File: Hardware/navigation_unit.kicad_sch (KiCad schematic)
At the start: 34 parts, among them SW1 SW_SPDT, SW2 SW_Push_Dual, U4 STM32F405RGTx, Y1 25MHz

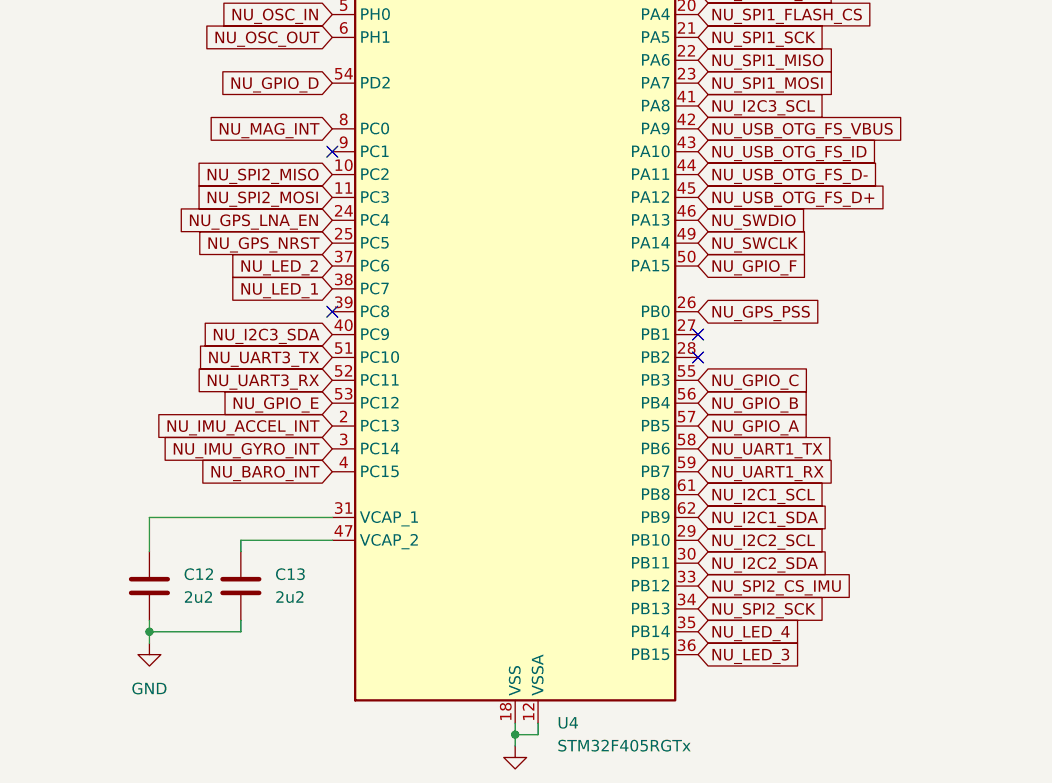
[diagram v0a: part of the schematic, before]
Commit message: i2c sensors traces
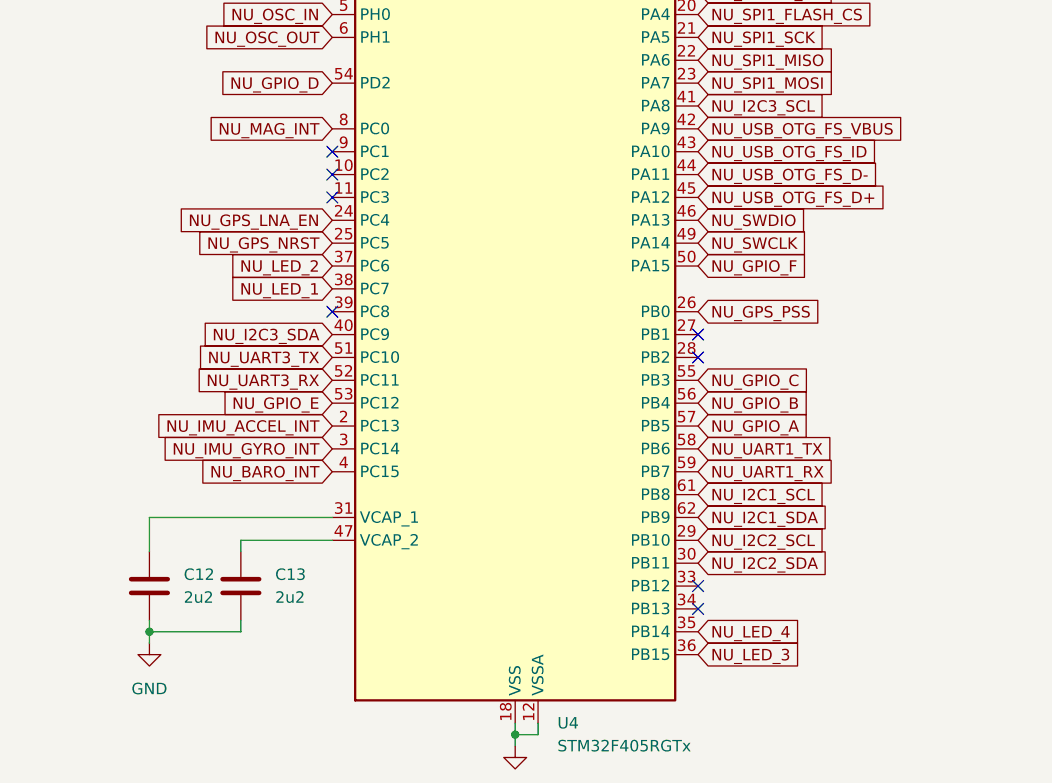
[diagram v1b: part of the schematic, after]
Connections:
- net NU_SPI2_CS_IMU: no longer names the net of U4.33 (PB12)
- net NU_SPI2_MISO: no longer names the net of U4.10 (PC2)
- net NU_SPI2_MOSI: no longer names the net of U4.11 (PC3)
- net NU_SPI2_SCK: no longer names the net of U4.34 (PB13)
- no-connect marks 4 -> 8
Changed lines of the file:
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@@
+	)
+	(no_connect
+		(at 90.17 143.51)
 	)
 	(no_connect
@@
 	)
 	(no_connect
+		(at 49.53 95.25)
+	)
+	(no_connect
 		(at 49.53 110.49)
 	)
+	(no_connect
+		(at 90.17 140.97)
+	)
+	(no_connect
+		(at 49.53 97.79)
+	)
 	(wire
 		(pts
@@
 		)
 	)
-	(global_label "NU_SPI2_CS_IMU"
-		(shape input)
-		(at 90.17 140.97 0)
-		(fields_autoplaced yes)
-		(effects
-			(font
-				(size 1.27 1.27)
-			)
-			(justify left)
-		)
-		(property "Intersheetrefs" "${INTERSHEET_REFS}"
-			(at 108.879 140.97 0)
-			(effects
-				(font
-					(size 1.27 1.27)
-				)
-				(justify left)
-				(hide yes)
-			)
-		)
-	)
 	(global_label "NU_USB_OTG_FS_D-"
 		(shape input)
@@
 		)
 	)
-	(global_label "NU_SPI2_SCK"
-		(shape input)
-		(at 90.17 143.51 0)
-		(fields_autoplaced yes)
-		(effects
-			(font
-				(size 1.27 1.27)
-			)
-			(justify left)
-		)
-		(property "Intersheetrefs" "${INTERSHEET_REFS}"
-			(at 105.7947 143.51 0)
-			(effects
-				(font
-					(size 1.27 1.27)
-				)
-				(justify left)
-				(hide yes)
-			)
-		)
-	)
 	(global_label "NU_I2C2_SDA"
 		(shape input)
@@
 		)
 	)
-	(global_label "NU_SPI2_MISO"
-		(shape input)
-		(at 49.53 95.25 180)
-		(fields_autoplaced yes)
-		(effects
-			(font
-				(size 1.27 1.27)
-			)
-			(justify right)
-		)
-		(property "Intersheetrefs" "${INTERSHEET_REFS}"
-			(at 33.0586 95.25 0)
-			(effects
-				(font
-					(size 1.27 1.27)
-				)
-				(justify right)
-				(hide yes)
-			)
-		)
-	)
 	(global_label "NU_SPI1_MISO"
 		(shape input)
@@
 				(hide yes)
 			)
-		)
-	)
-	(global_label "NU_SPI2_MOSI"
-		(shape input)
-		(at 49.53 97.79 180)
-		(fields_autoplaced yes)
-		(effects
-			(font
-				(size 1.27 1.27)
-			)
-			(justify right)
-		)
-		(property "Intersheetrefs" "${INTERSHEET_REFS}"
-			(at 33.0586 97.79 0)
-			(effects
-				(font
-					(size 1.27 1.27)
-				)
-				(justify right)
-				(hide yes)
-			)
